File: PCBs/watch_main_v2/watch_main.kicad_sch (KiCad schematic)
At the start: 1 part, among them U101 Watch_Outline_V2

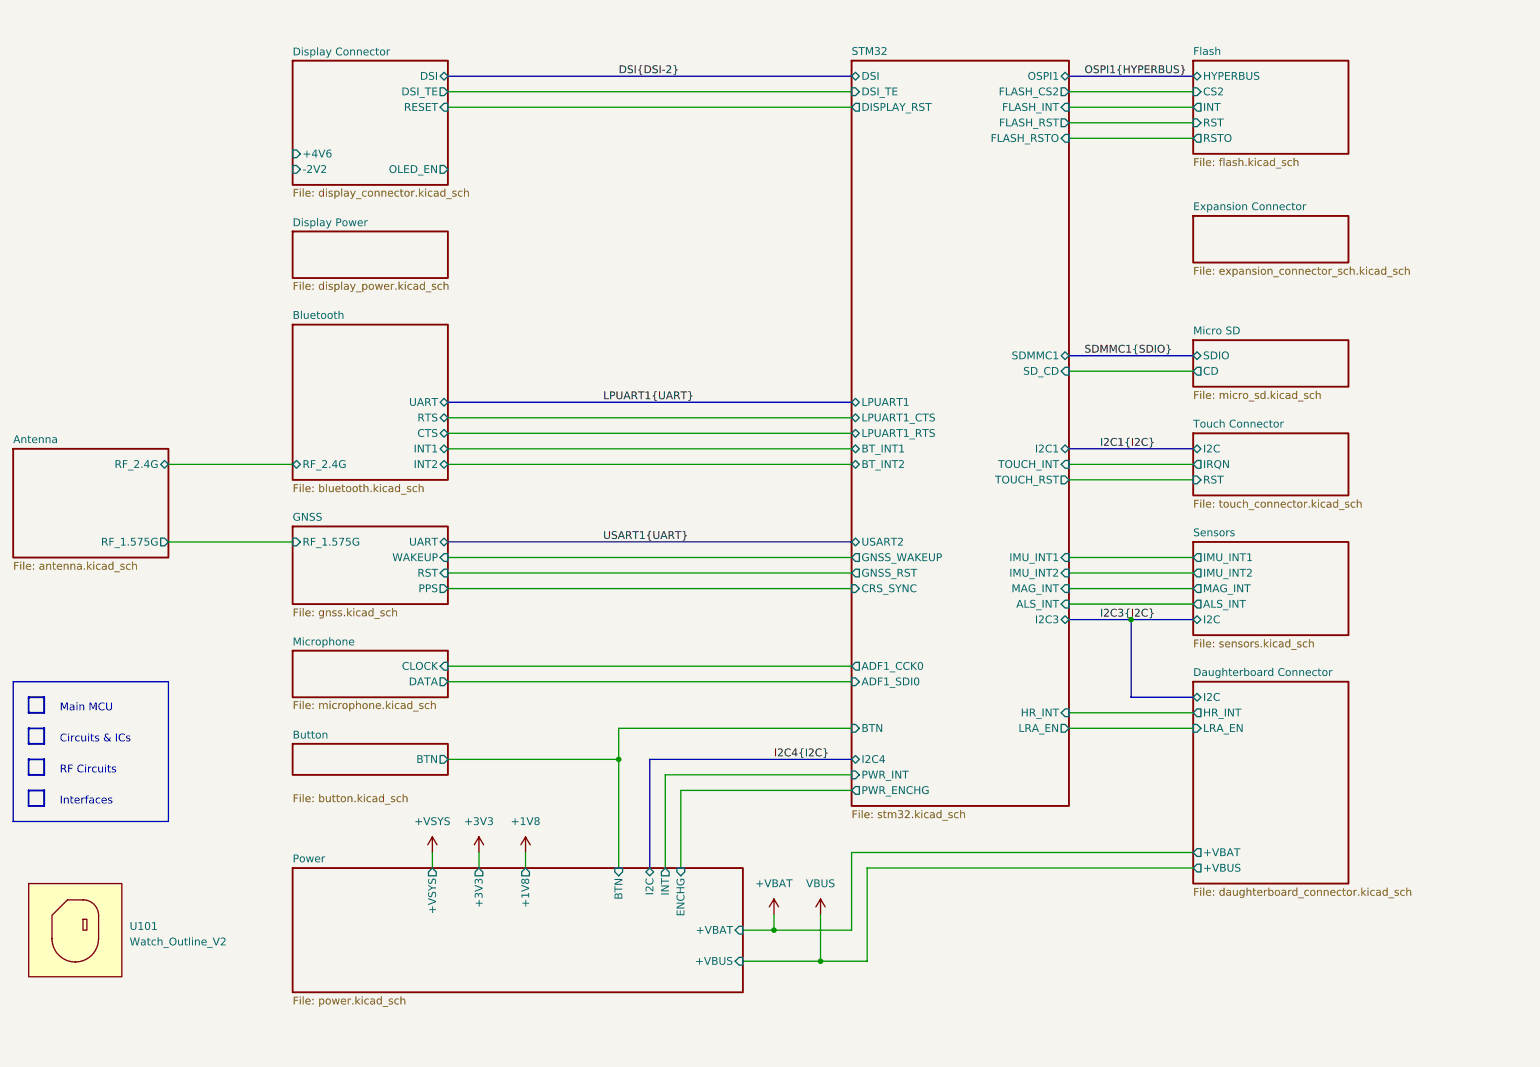
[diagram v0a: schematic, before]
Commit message: Schematic v2 complete
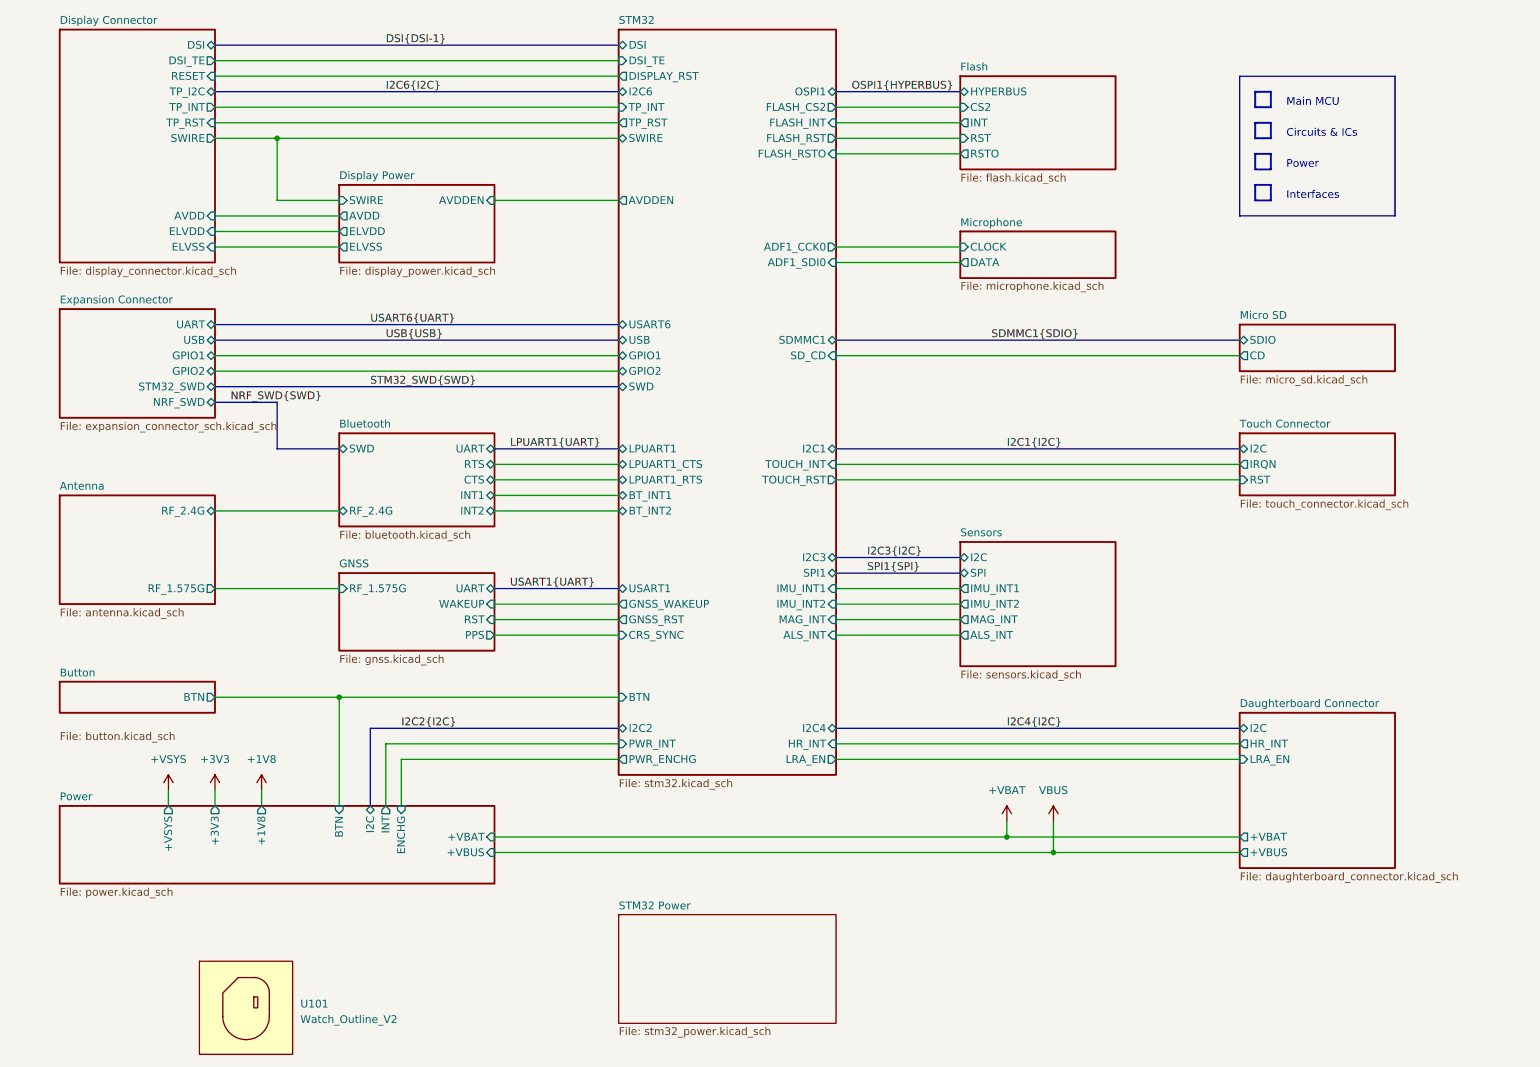
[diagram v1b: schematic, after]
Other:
- added sheet STM32 Power (stm32_power.kicad_sch)
- sheet Bluetooth ports: added SWD; removed none
- sheet Display Connector ports: added AVDD, ELVDD, ELVSS, SWIRE, TP_I2C, TP_INT, TP_RST; removed +4V6, -2V2, OLED_EN
- sheet Display Power ports: added AVDD, AVDDEN, ELVDD, ELVSS, SWIRE; removed none
- sheet Expansion Connector ports: added GPIO1, GPIO2, NRF_SWD, STM32_SWD, UART, USB; removed none
- sheet STM32 ports: added AVDDEN, GPIO1, GPIO2, I2C2, I2C6, SPI1, SWD, SWIRE, TP_INT, TP_RST, USART1, USART6, USB; removed USART2
- sheet Sensors ports: added SPI; removed none
- note added: "Power"
- note removed: "RF Circuits"
- moved on the sheet: U101
